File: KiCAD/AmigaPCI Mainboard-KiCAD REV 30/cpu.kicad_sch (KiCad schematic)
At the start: 49 parts, among them CN712 SPI, U200 MC68040, U712 ICE40HX4K-TQ144, U712F1 W25X20CLSN

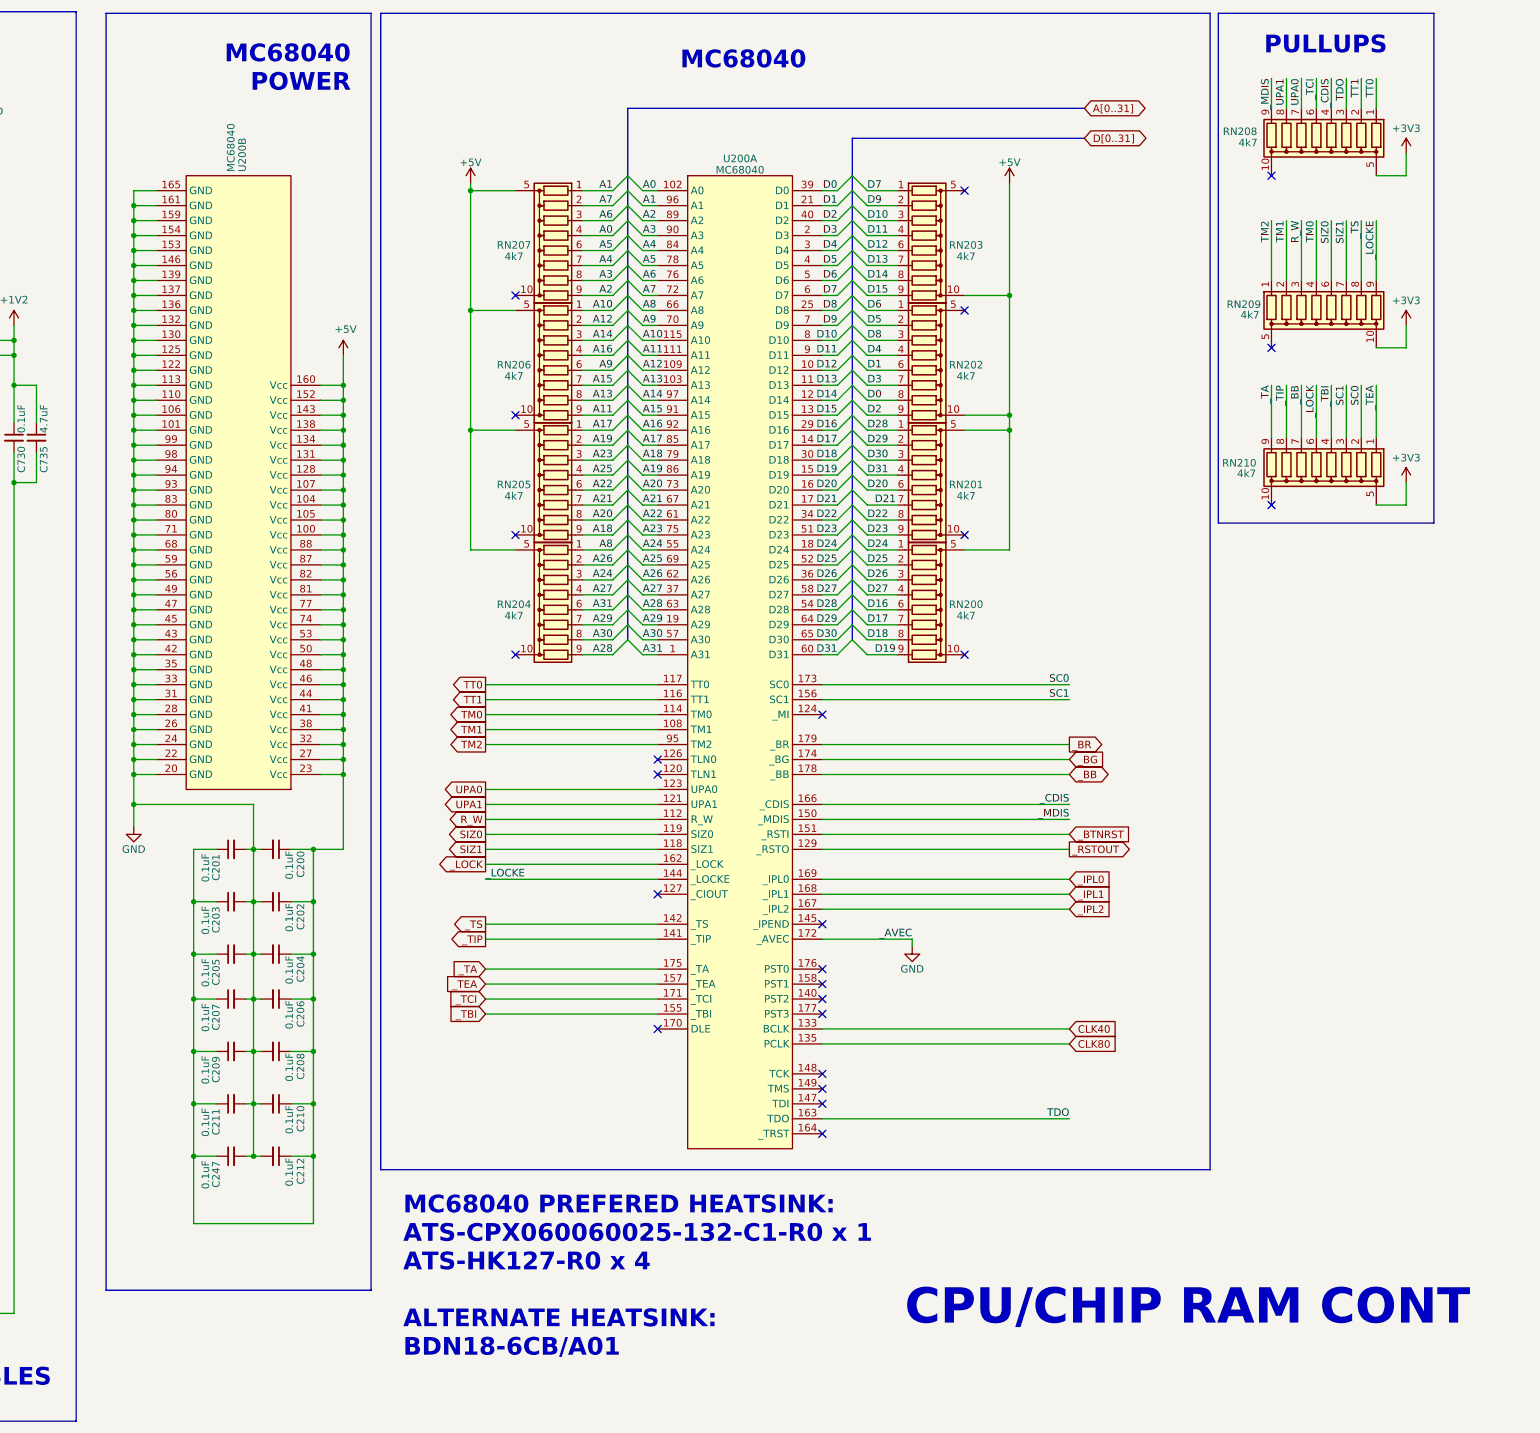
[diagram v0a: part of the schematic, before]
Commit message: Rev 3.0 PCB Routing 12-MAY-2024
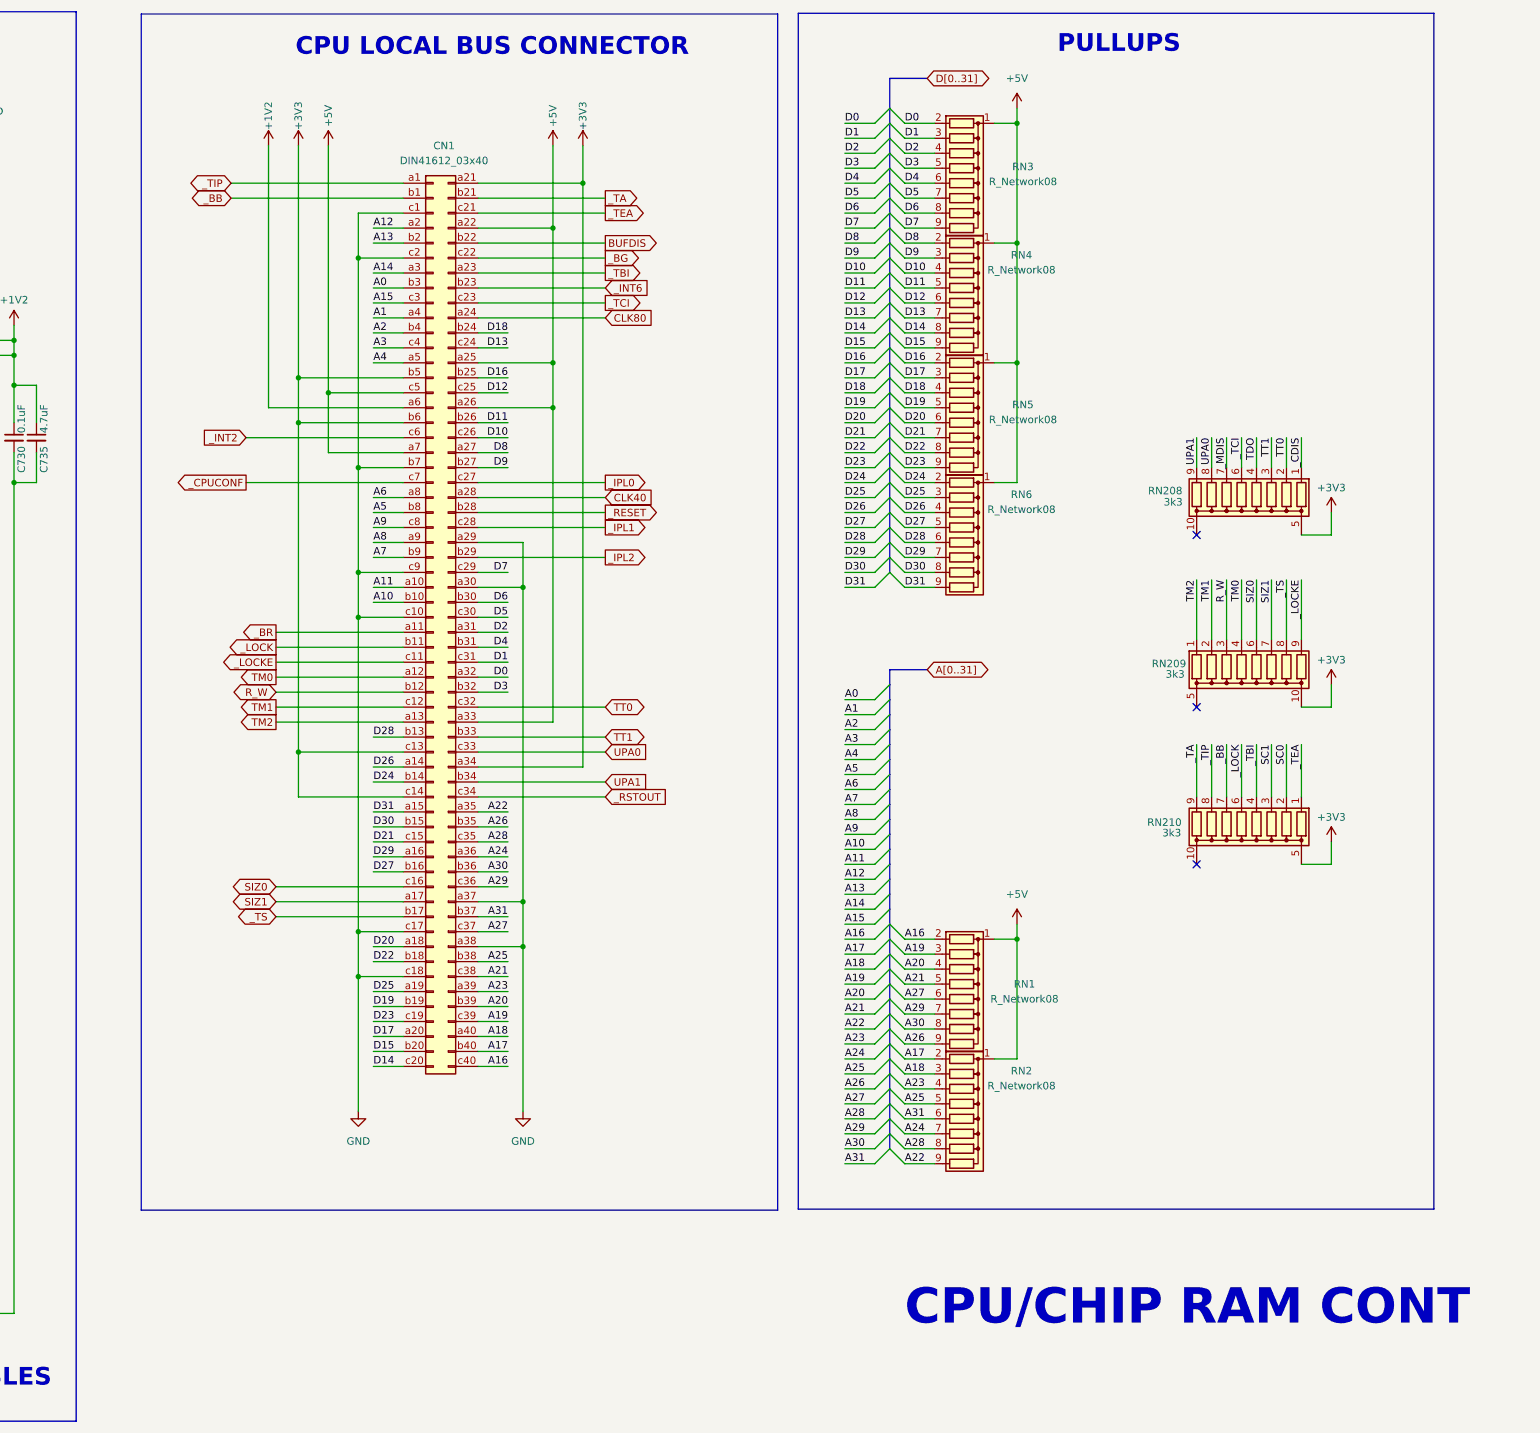
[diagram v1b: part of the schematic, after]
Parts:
- removed C200, C201, C202, C203, C204, C205, C206, C207, C208, C209, C210, C211, C212, C247: 0.1uF, Capacitor_SMD:C_0603_1608Metric, symbol Device:C_Small
- removed RN200, RN201, RN202, RN203, RN204, RN205, RN206, RN207: 4k7, Resistor_SMD:R_Array_Convex_5x1206, symbol AmigaPCI-Symbols:R_SM_Network08
- removed U200: MC68040, AmigaPCI:PGA179, symbol AmigaPCI-Symbols:MC68040RC33
- added CN1: DIN41612_03x40, AmigaPCI:DIN41612_C_3x40_Female_Vertical_THT, symbol AmigaPCI-Symbols:DIN41612_03x40
- added RN1, RN2, RN3, RN4, RN5, RN6: R_Network08, Resistor_THT:R_Array_SIP9, symbol Device:R_Network08
- RN208, RN209, RN210: value 4k7 -> 3k3; footprint Resistor_SMD:R_Array_Convex_5x1206 -> Resistor_SMD:R_Array_Convex_5x0603; Part YC358TJK-074K7L -> YC158TJR-073K3L
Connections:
- net +1V2: now also CN1.a6 (Pin_a6)
- net +3V3: now also CN1.a21 (Pin_a21), CN1.a34 (Pin_a34), CN1.b5 (Pin_b5), CN1.b6 (Pin_b6), CN1.c13 (Pin_c13), CN1.c14 (Pin_c14)
- net +5V: now also CN1.a22 (Pin_a22), CN1.a25 (Pin_a25), CN1.a26 (Pin_a26), CN1.a33 (Pin_a33), CN1.a7 (Pin_a7), CN1.c5 (Pin_c5), RN1.1 (common), RN2.1 (common), RN3.1 (common), RN4.1 (common), RN5.1 (common), RN6.1 (common)
- net A0: now also CN1.b3 (Pin_b3)
- net A1: now also CN1.a4 (Pin_a4)
- net A10: now also CN1.b10 (Pin_b10)
- net A11: now also CN1.a10 (Pin_a10)
- net A12: now also CN1.a2 (Pin_a2)
- net A13: now also CN1.b2 (Pin_b2)
- net A14: now also CN1.a3 (Pin_a3)
- net A15: now also CN1.c3 (Pin_c3)
- net A16: now also CN1.c40 (Pin_c40), RN1.2 (R1)
- net A17: now also CN1.b40 (Pin_b40), RN2.2 (R1)
- net A18: now also CN1.a40 (Pin_a40), RN2.3 (R2)
- net A19: now also CN1.c39 (Pin_c39), RN1.3 (R2)
- net A2: now also CN1.b4 (Pin_b4)
- net A20: now also CN1.b39 (Pin_b39), RN1.4 (R3)
- net A21: now also CN1.c38 (Pin_c38), RN1.5 (R4)
- net A22: now also CN1.a35 (Pin_a35), RN2.9 (R8)
- net A23: now also CN1.a39 (Pin_a39), RN2.4 (R3)
- net A24: now also CN1.a36 (Pin_a36), RN2.7 (R6)
- net A25: now also CN1.b38 (Pin_b38), RN2.5 (R4)
- net A26: now also CN1.b35 (Pin_b35), RN1.9 (R8)
- net A27: now also CN1.c37 (Pin_c37), RN1.6 (R5)
- net A28: now also CN1.c35 (Pin_c35), RN2.8 (R7)
- net A29: now also CN1.c36 (Pin_c36), RN1.7 (R6)
- net A3: now also CN1.c4 (Pin_c4)
- net A30: now also CN1.b36 (Pin_b36), RN1.8 (R7)
- net A31: now also CN1.b37 (Pin_b37), RN2.6 (R5)
- net A4: now also CN1.a5 (Pin_a5)
- net A5: now also CN1.b8 (Pin_b8)
- net A6: now also CN1.a8 (Pin_a8)
- net A7: now also CN1.b9 (Pin_b9)
- net A8: now also CN1.a9 (Pin_a9)
- net A9: now also CN1.c8 (Pin_c8)
- net CLK40: now also CN1.a28 (Pin_a28)
- net CLK80: now also CN1.a24 (Pin_a24)
- net D0: now also CN1.a32 (Pin_a32), RN3.2 (R1)
- net D1: now also CN1.c31 (Pin_c31), RN3.3 (R2)
- net D10: now also CN1.c26 (Pin_c26), RN4.4 (R3)
- net D11: now also CN1.b26 (Pin_b26), RN4.5 (R4)
- net D12: now also CN1.c25 (Pin_c25), RN4.6 (R5)
- net D13: now also CN1.c24 (Pin_c24), RN4.7 (R6)
- net D14: now also CN1.c20 (Pin_c20), RN4.8 (R7)
- net D15: now also CN1.b20 (Pin_b20), RN4.9 (R8)
- net D16: now also CN1.b25 (Pin_b25), RN5.2 (R1)
- net D17: now also CN1.a20 (Pin_a20), RN5.3 (R2)
- net D18: now also CN1.b24 (Pin_b24), RN5.4 (R3)
- net D19: now also CN1.b19 (Pin_b19), RN5.5 (R4)
- net D2: now also CN1.a31 (Pin_a31), RN3.4 (R3)
- net D20: now also CN1.a18 (Pin_a18), RN5.6 (R5)
- net D21: now also CN1.c15 (Pin_c15), RN5.7 (R6)
- net D22: now also CN1.b18 (Pin_b18), RN5.8 (R7)
- net D23: now also CN1.c19 (Pin_c19), RN5.9 (R8)
- net D24: now also CN1.b14 (Pin_b14), RN6.2 (R1)
- net D25: now also CN1.a19 (Pin_a19), RN6.3 (R2)
- net D26: now also CN1.a14 (Pin_a14), RN6.4 (R3)
- net D27: now also CN1.b16 (Pin_b16), RN6.5 (R4)
- net D28: now also CN1.b13 (Pin_b13), RN6.6 (R5)
- net D29: now also CN1.a16 (Pin_a16), RN6.7 (R6)
- net D3: now also CN1.b32 (Pin_b32), RN3.5 (R4)
- net D30: now also CN1.b15 (Pin_b15), RN6.8 (R7)
- net D31: now also CN1.a15 (Pin_a15), RN6.9 (R8)
- net D4: now also CN1.b31 (Pin_b31), RN3.6 (R5)
- net D5: now also CN1.c30 (Pin_c30), RN3.7 (R6)
- net D6: now also CN1.b30 (Pin_b30), RN3.8 (R7)
- net D7: now also CN1.c29 (Pin_c29), RN3.9 (R8)
- net D8: now also CN1.a27 (Pin_a27), RN4.2 (R1)
- net D9: now also CN1.b27 (Pin_b27), RN4.3 (R2)
- net GND: now also CN1.a29 (Pin_a29), CN1.a30 (Pin_a30), CN1.a37 (Pin_a37), CN1.a38 (Pin_a38), CN1.b7 (Pin_b7), CN1.c1 (Pin_c1), CN1.c10 (Pin_c10), CN1.c17 (Pin_c17), CN1.c18 (Pin_c18), CN1.c2 (Pin_c2), CN1.c9 (Pin_c9)
- net R_W: now also CN1.b12 (Pin_b12)
- net SIZ0: now also CN1.c16 (Pin_c16)
- net SIZ1: now also CN1.a17 (Pin_a17)
- net TDO: now also RN208.4 (R4); no longer RN208.3 (R3)
- net TM0: now also CN1.a12 (Pin_a12)
- net TM1: now also CN1.c12 (Pin_c12)
- net TM2: now also CN1.a13 (Pin_a13)
- net TT0: now also RN208.2 (R2), CN1.c32 (Pin_c32); no longer RN208.1 (R1)
- net TT1: now also RN208.3 (R3), CN1.b33 (Pin_b33); no longer RN208.2 (R2)
- net UPA0: now also RN208.8 (R7), CN1.c33 (Pin_c33); no longer RN208.7 (R6)
- net UPA1: now also RN208.9 (R8), CN1.b34 (Pin_b34); no longer RN208.8 (R7)
- net _BB: now also CN1.b1 (Pin_b1)
- net _BG: now also CN1.c22 (Pin_c22)
- net _BR: now also CN1.a11 (Pin_a11)
- net _CDIS: now also RN208.1 (R1); no longer RN208.4 (R4)
- net _IPL0: now also CN1.c27 (Pin_c27)
- net _IPL1: now also CN1.c28 (Pin_c28)
- net _IPL2: now also CN1.b29 (Pin_b29)
- net _LOCK: now also CN1.b11 (Pin_b11)
- net _LOCKE: now also CN1.c11 (Pin_c11)
- net _MDIS: now also RN208.7 (R6); no longer RN208.9 (R8)
- net _RESET: now also CN1.b28 (Pin_b28)
- net _RSTOUT: now also CN1.c34 (Pin_c34)
- net _TA: now also CN1.b21 (Pin_b21)
- net _TBI: now also CN1.a23 (Pin_a23)
- net _TCI: now also CN1.c23 (Pin_c23)
- net _TEA: now also CN1.c21 (Pin_c21)
- net _TIP: now also CN1.a1 (Pin_a1)
- net _TS: now also CN1.b17 (Pin_b17)
- new net BUFDIS: CN1.b22 (Pin_b22)
- new net _CPUCONF: CN1.c7 (Pin_c7)
- new net _INT2: CN1.c6 (Pin_c6)
- new net _INT6: CN1.b23 (Pin_b23)
- no-connect marks 35 -> 13
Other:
- note added: "CPU LOCAL BUS CONNECTOR"
- note removed: "MC68040"
- note removed: "MC68040 POWER"
- note removed: "MC68040 PREFERED HEATSINK: ATS-CPX060060025-132-C1-R0 x 1 ATS-HK127-R0 x 4 ALTERNATE HEATSINK: BDN18-6CB/A01"
- moved on the sheet: RN208, RN209, RN210
